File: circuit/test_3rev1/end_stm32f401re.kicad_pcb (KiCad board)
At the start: 2 copper layers, 61 x 88.9 mm, 67 parts, among them J2 USB_B_Micro, U1 MAX98357, U2 STM32F401RETx, U3 AMS1117-3.3, U4 MAX98357, U5 ESP-12E

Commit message: update PCB
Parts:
- L-DACN1, L-DACN2, L-DACP1, L-DACP2: value L -> 100uH
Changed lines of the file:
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@@
   )
   (setup
-    (last_trace_width 0.3)
+    (last_trace_width 0.25)
     (user_trace_width 0.3)
     (user_trace_width 0.4)
@@
       (effects (font (size 1 1) (thickness 0.15)))
     )
-    (fp_text value L (at 0 1.65 90) (layer F.Fab)
+    (fp_text value 100uH (at 0 1.65 90) (layer F.Fab)
       (effects (font (size 1 1) (thickness 0.15)))
     )
@@
       (effects (font (size 1 1) (thickness 0.15)))
     )
-    (fp_text value L (at 0 1.65 90) (layer F.Fab)
+    (fp_text value 100uH (at 0 1.65 90) (layer F.Fab)
       (effects (font (size 1 1) (thickness 0.15)))
     )
@@
       (effects (font (size 1 1) (thickness 0.15)))
     )
-    (fp_text value L (at 0 1.65 90) (layer F.Fab)
+    (fp_text value 100uH (at 0 1.65 90) (layer F.Fab)
       (effects (font (size 1 1) (thickness 0.15)))
     )
@@
       (effects (font (size 1 1) (thickness 0.15)))
     )
-    (fp_text value L (at 0 1.65 90) (layer F.Fab)
-      (effects (font (size 1 1) (thickness 0.15)))
-    )
+    (fp_text value 100uH (at 0 1.65 90) (layer F.Fab)
+      (effects (font (size 1 1) (thickness 0.15)))
+    )

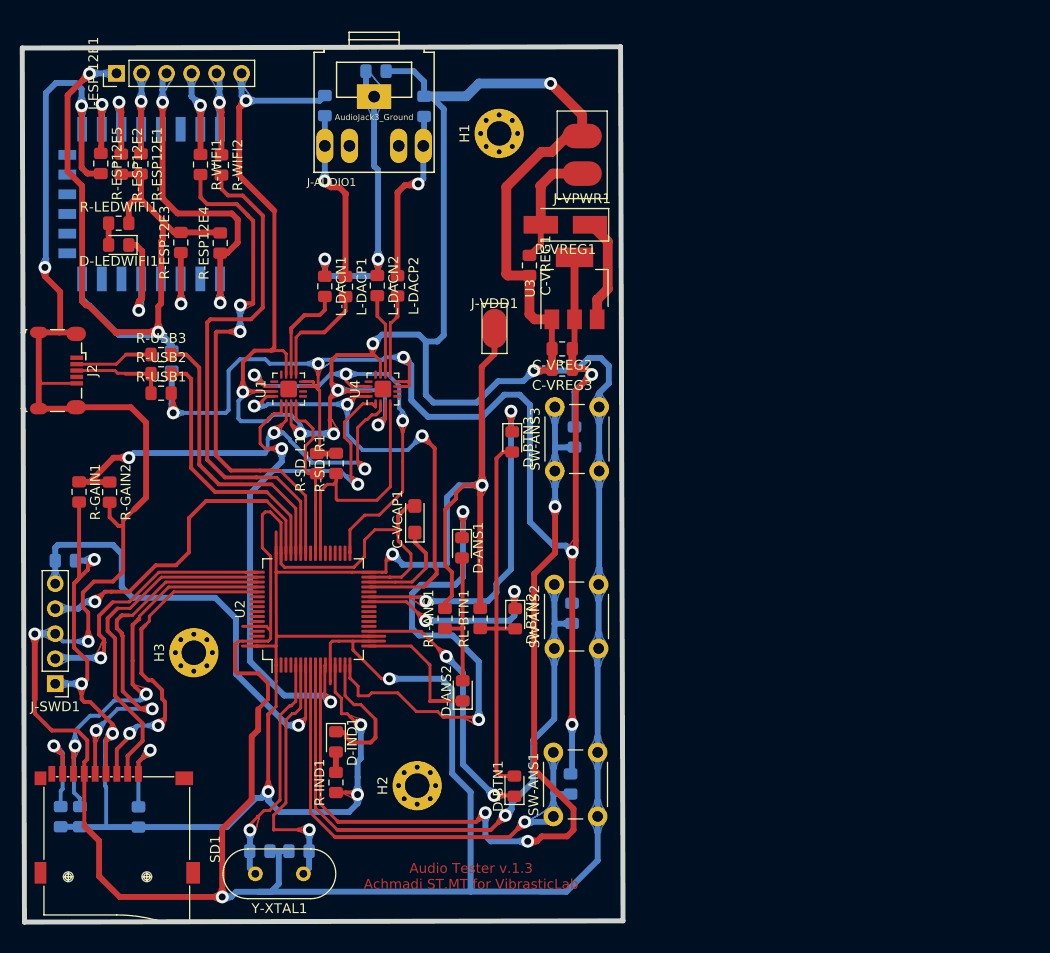
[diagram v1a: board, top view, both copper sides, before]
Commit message: reset button
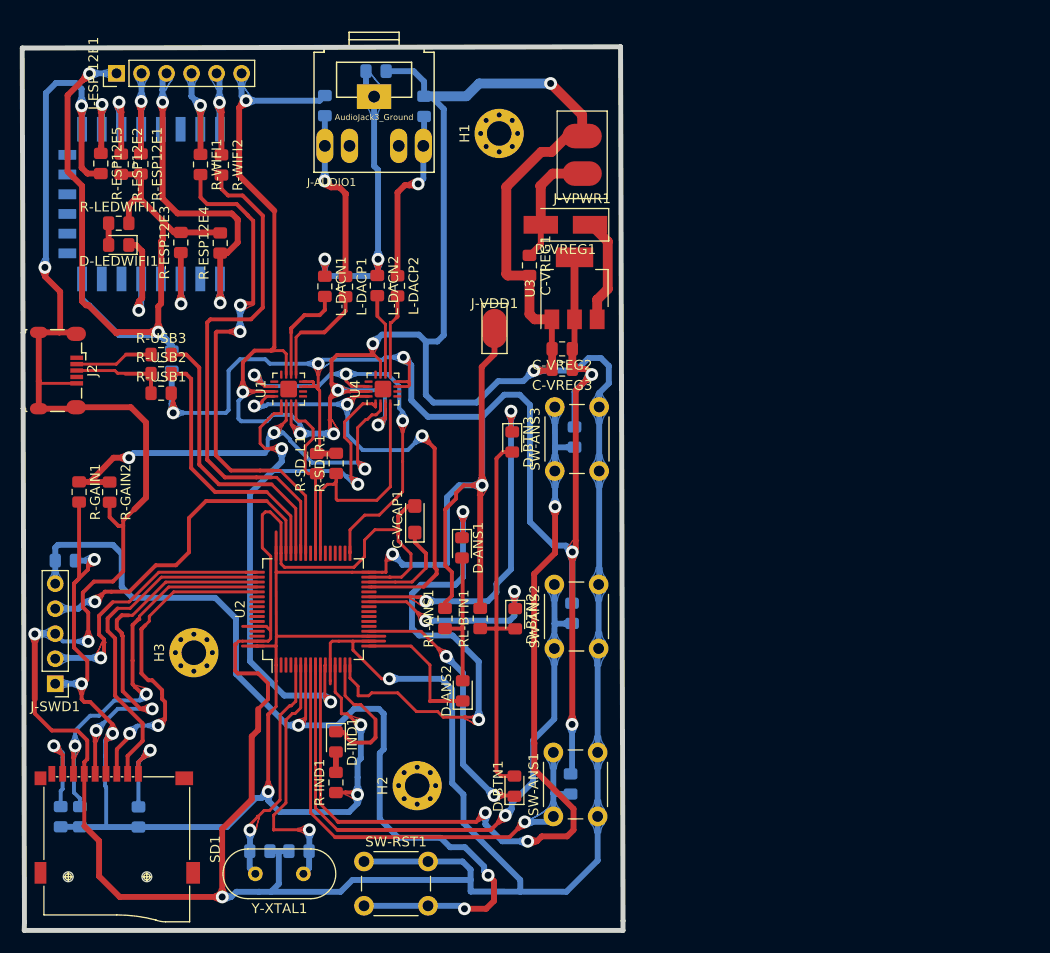
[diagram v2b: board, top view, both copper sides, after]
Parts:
- added SW-RST1: SW_Push, Button_Switch_THT:SW_PUSH_6mm, F.Cu at (84.2, 108.0)
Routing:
- net /NRST: track 47.8 -> 98.3 mm, vias 1 -> 3
- net GND: track 592.8 -> 607.6 mm
- net /BTN_C: track 91.5 -> 90.8 mm
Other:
- board size 61 x 88.9 mm -> 61 x 89.7 mm
- board text removed: "Audio Tester v.1.3 Achmadi ST.MT for VibrasticLab"

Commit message: new PCB
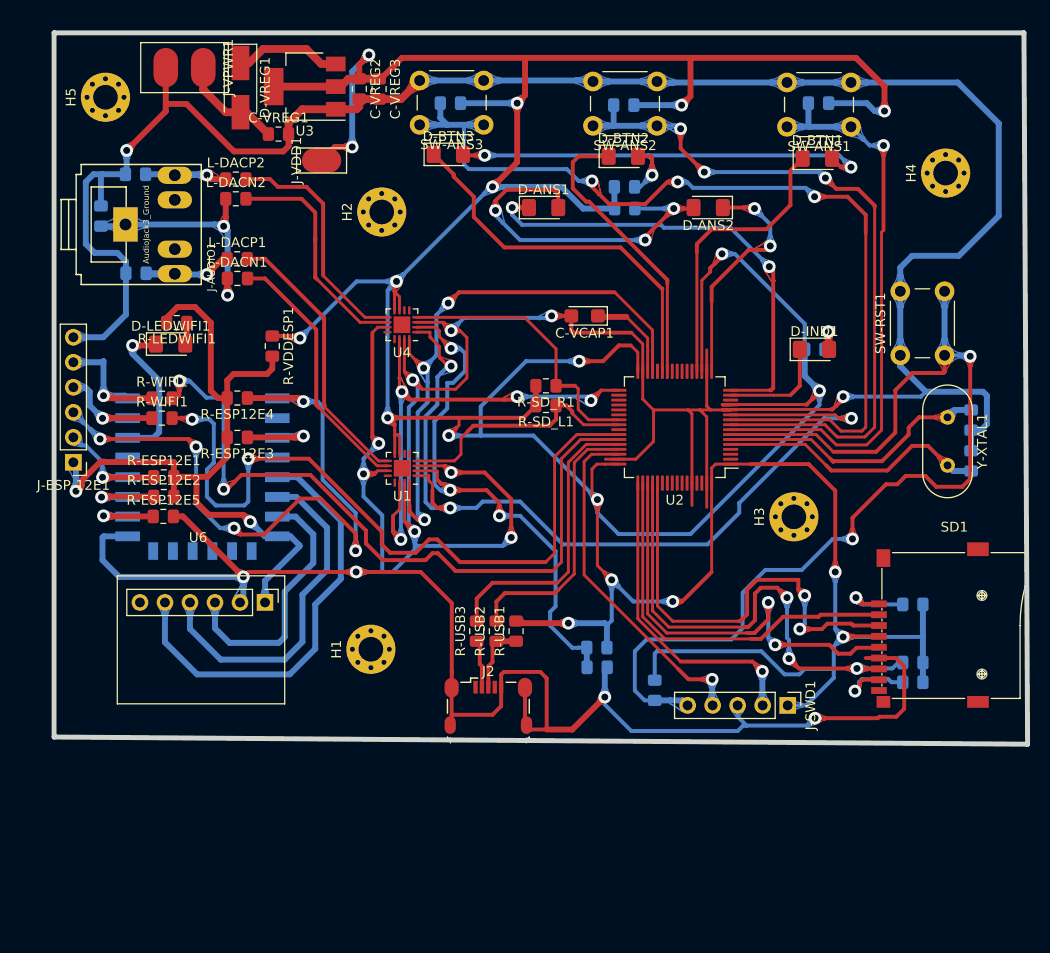
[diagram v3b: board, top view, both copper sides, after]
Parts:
- removed G***: LOGO, viblab:viblab
- added H4: MountingHole, MountingHole:MountingHole_2.5mm_Pad_Via, F.Cu at (143.3, 38.1)
- added H5: CableHole, MountingHole:MountingHole_2.5mm_Pad_Via, F.Cu at (58.0, 30.4)
- added U6: SPH0645, mic:sph0645, F.Cu at (67.3, 82.3)
- D-ANS1, D-ANS2, D-BTN1, D-BTN2, D-BTN3, D-IND1, D-LEDWIFI1: footprint LED_SMD:LED_0805_2012Metric_Pad1.15x1.40mm_HandSolder -> LED_SMD:LED_1206_3216Metric_Pad1.42x1.75mm_HandSolder
- R-GAIN1, R-GAIN2, R-IND1, RL-ANS1, RL-BTN1: moved to B.Cu
- R-VDDESP1: moved to F.Cu
- moved SD1 88.1 mm to (144.2, 84.0), turned to 0 degrees
- moved R-SD3 87.6 mm to (139.9, 89.8), turned to 0 degrees
- moved R-SD2 86.0 mm to (139.9, 87.8), turned to 0 degrees
- moved C-XTAL1 82.4 mm to (145.8, 67.3), turned to 90 degrees
- moved R-SD1 81.5 mm to (139.9, 81.9), turned to 0 degrees
- moved C-XTAL2 81.1 mm to (145.8, 63.2), turned to 270 degrees
- moved Y-XTAL1 80.2 mm to (143.4, 62.9), turned to 270 degrees
- moved SW-ANS1 76.3 mm to (133.7, 33.4), turned to 180 degrees
- moved SW-RST1 74.9 mm to (138.7, 56.6), turned to 90 degrees
- moved J-SWD1 74.4 mm to (127.2, 92.2), turned to 270 degrees
- moved R-ANS1 73.6 mm to (130.3, 31.0), turned to 180 degrees
- moved D-BTN1 70.8 mm to (130.2, 36.6), turned to 0 degrees
- moved R-IND1 65.6 mm to (130.0, 56.0), turned to 0 degrees
- moved D-IND1 62.8 mm to (129.9, 56.0), turned to 0 degrees
- moved H3 62.5 mm to (127.8, 73.0)
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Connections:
- U5 pad 20: Net-(U5-Pad20) -> /ESP_LEDWIFI
- U5 pad 5: /ESP_LEDWIFI -> /MIC_LRCL
- U5 pad 6: Net-(U5-Pad6) -> /MIC_DOUT
- U5 pad 7: Net-(U5-Pad7) -> /MIC_BCLK
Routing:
- net VDD: track 381.0 -> 461.5 mm, vias 14 -> 19
- net GND: track 607.6 -> 535.1 mm, vias 15 -> 14
- net /MIC_LRCL: track 0.00 -> 44.1 mm
- net /MIC_DOUT: track 0.00 -> 35.1 mm
- net /ESP_RST: track 35.4 -> 68.8 mm, vias 2 -> 5
- net /MIC_BCLK: track 0.00 -> 26.6 mm
- net /DAC_DIN: track 65.8 -> 91.0 mm
- net /WIFI_TXD: track 52.8 -> 76.4 mm
- net Net-(D-ANS1-Pad2): track 14.3 -> 36.6 mm, vias 0 -> 3
- net /WIFI_RXD: track 52.8 -> 74.6 mm, vias 0 -> 2
- net Net-(L-DACP1-Pad2): track 11.4 -> 28.0 mm
- net Net-(L-DACN1-Pad2): track 10.3 -> 26.6 mm
- net Net-(L-DACP2-Pad2): track 8.36 -> 24.5 mm
- net Net-(L-DACN2-Pad2): track 8.35 -> 23.7 mm
- net /MMC_MOSI: track 32.8 -> 44.5 mm
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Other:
- board size 61 x 89.7 mm -> 98.9 x 72.2 mm
